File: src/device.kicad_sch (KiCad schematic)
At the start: 68 parts, among them J1 CN-REMO_3W, U1 TLIN14313-Q1, U2 nRF54L10-QDAA, Y1 32MHz, Y2 32.768kHz

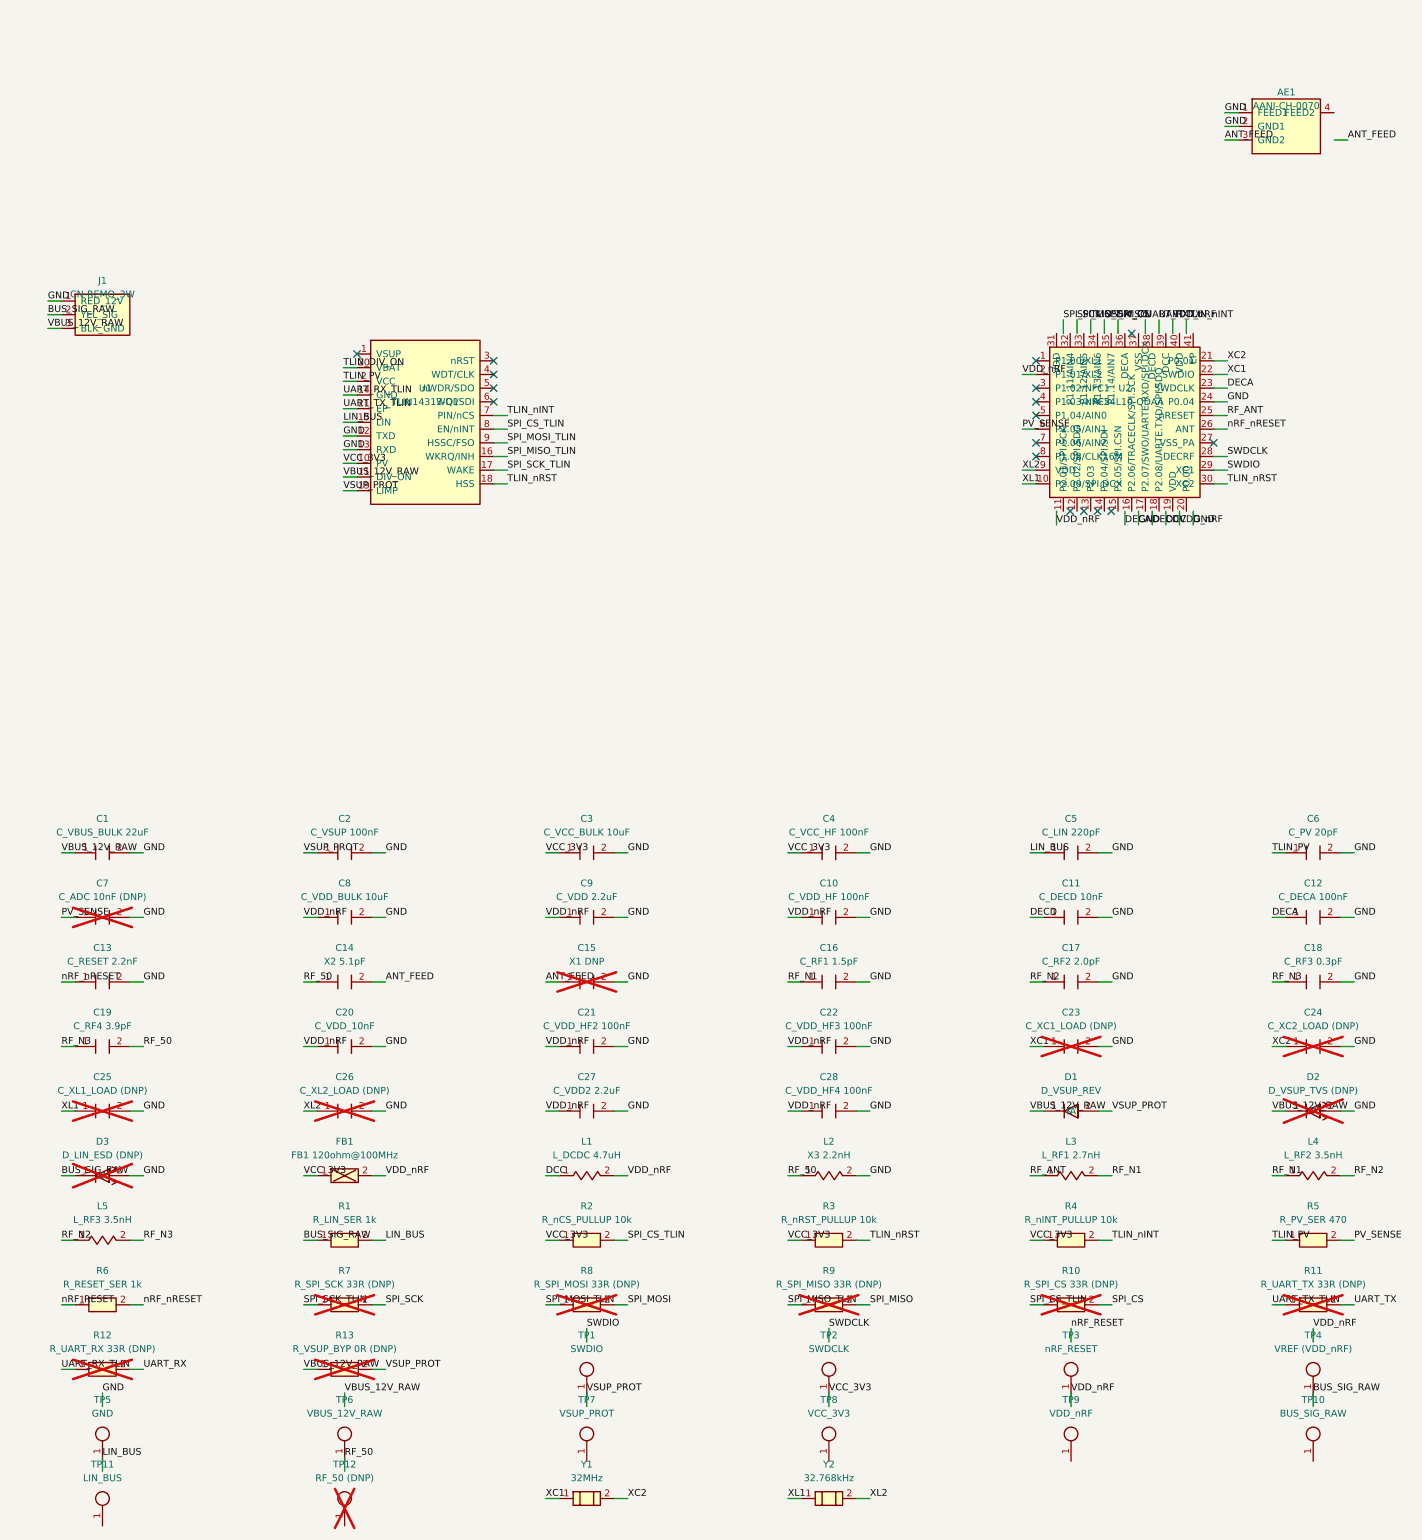
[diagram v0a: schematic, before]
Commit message: stage
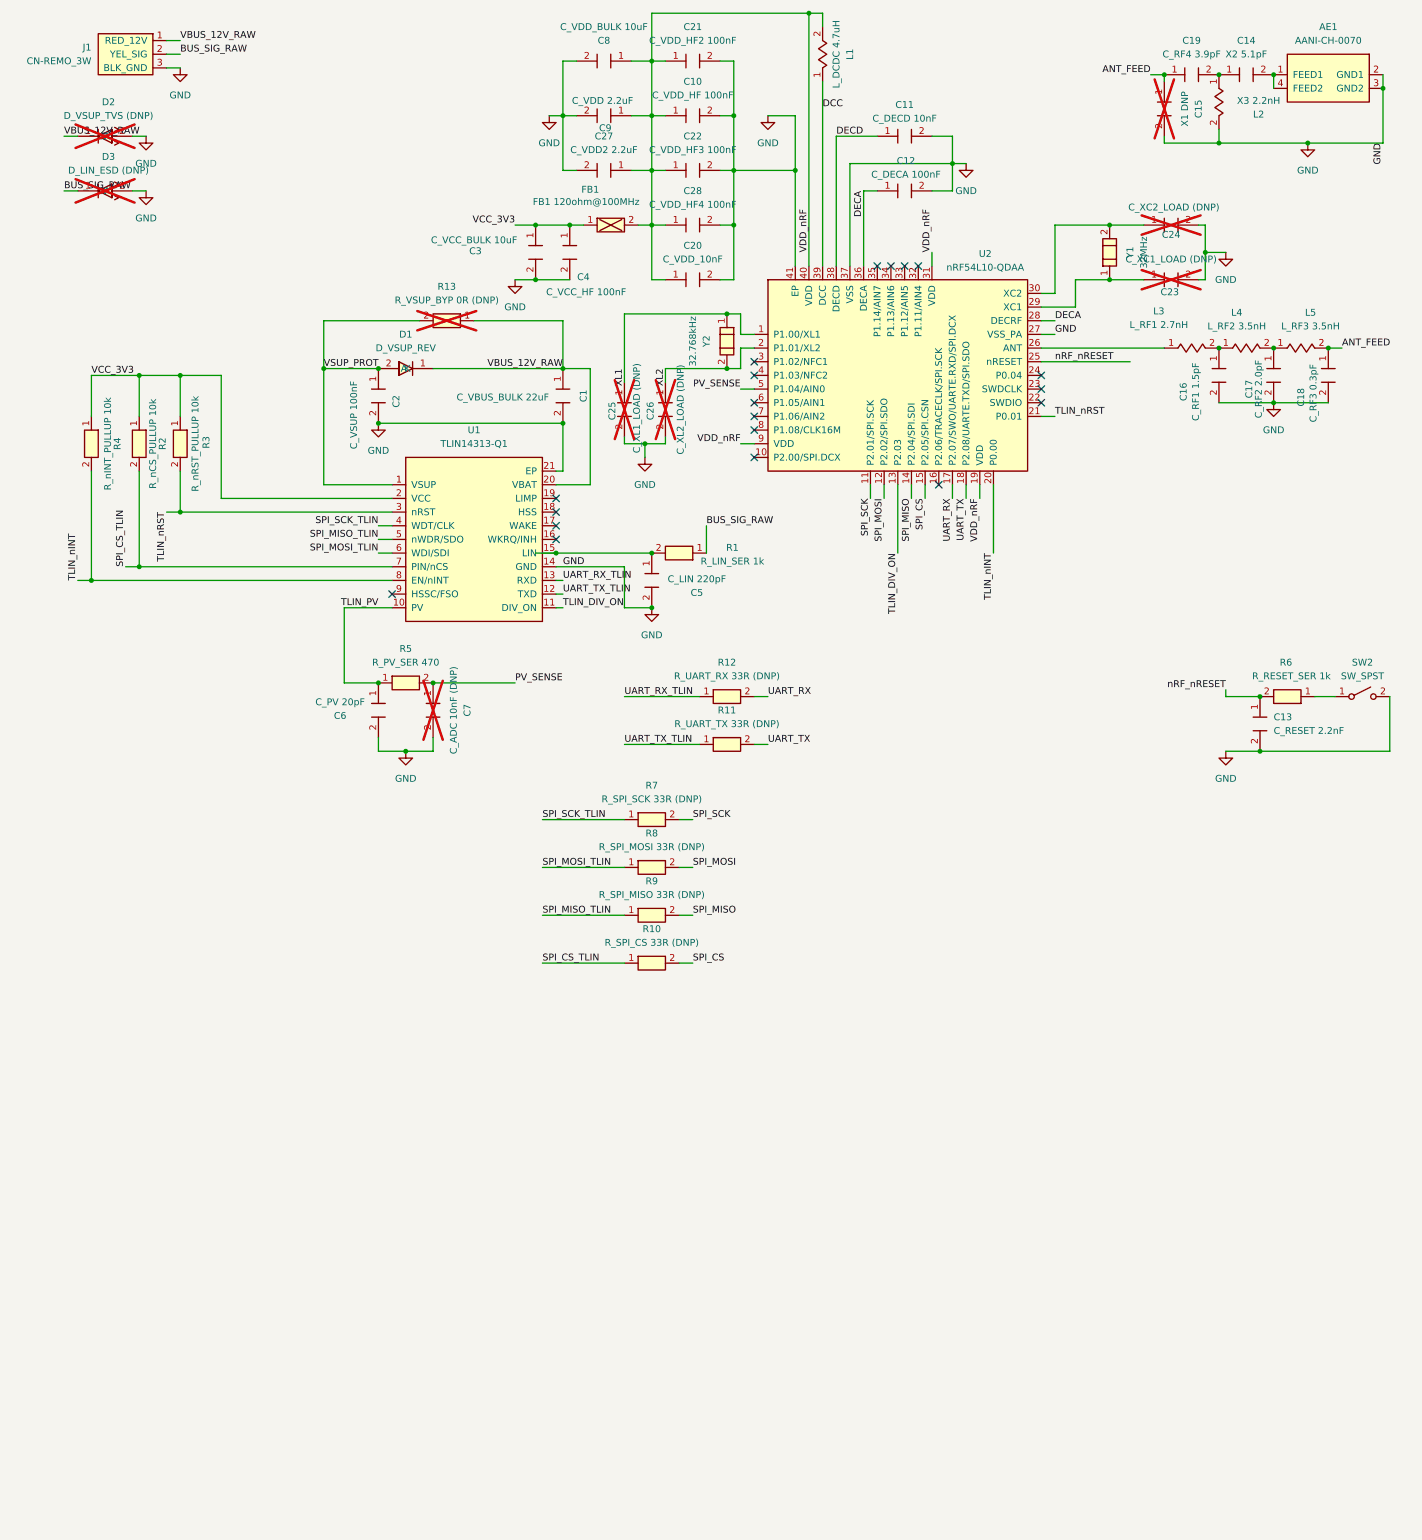
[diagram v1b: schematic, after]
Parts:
- removed TP1: SWDIO, TestPoint:TestPoint_Pad_D1.0mm, symbol device:TestPoint
- removed TP10: BUS_SIG_RAW, TestPoint:TestPoint_Pad_D1.0mm, symbol device:TestPoint
- removed TP11: LIN_BUS, TestPoint:TestPoint_Pad_D1.0mm, symbol device:TestPoint
- removed TP12: RF_50 (DNP), TestPoint:TestPoint_Pad_D1.0mm, symbol device:TestPoint
- removed TP2: SWDCLK, TestPoint:TestPoint_Pad_D1.0mm, symbol device:TestPoint
- removed TP3: nRF_RESET, TestPoint:TestPoint_Pad_D1.0mm, symbol device:TestPoint
- removed TP4: VREF (VDD_nRF), TestPoint:TestPoint_Pad_D1.0mm, symbol device:TestPoint
- removed TP5: GND, TestPoint:TestPoint_Pad_D1.0mm, symbol device:TestPoint
- removed TP6: VBUS_12V_RAW, TestPoint:TestPoint_Pad_D1.0mm, symbol device:TestPoint
- removed TP7: VSUP_PROT, TestPoint:TestPoint_Pad_D1.0mm, symbol device:TestPoint
- removed TP8: VCC_3V3, TestPoint:TestPoint_Pad_D1.0mm, symbol device:TestPoint
- removed TP9: VDD_nRF, TestPoint:TestPoint_Pad_D1.0mm, symbol device:TestPoint
- added SW2: SW_SPST, symbol Switch:SW_SPST
- R10, R11, R12, R7, R8, R9: now fitted
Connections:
- net RF_N3 is gone; now on net ANT_FEED: C18.1, C19.1, L5.2
- net SWDCLK is gone; now on net DECA: U2.28 (DECRF)
- net ANT_FEED: no longer AE1.3 (GND2), C14.2
- net DCC: now also U2.39 (DCC)
- net DECA: now also U2.36 (DECA); no longer U2.23 (SWDCLK)
- net DECD: now also U2.38 (DECD)
- net GND: now also AE1.3 (GND2), J1.3 (BLK_GND), U1.14 (GND), U1.21 (EP), U2.27 (VSS_PA), U2.37 (VSS), U2.41 (EP), SW2.2 (B); no longer AE1.1 (FEED1), J1.1 (RED_12V), U1.12 (TXD), U1.13 (RXD), U2.24 (P0.04)
- net PV_SENSE: now also U2.5 (P1.04/AIN0); no longer U2.6 (P1.05/AIN1)
- net SPI_CS: now also U2.15 (P2.05/SPI.CSN)
- net SPI_CS_TLIN: now also U1.7 (PIN/nCS); no longer U1.8 (EN/nINT)
- net SPI_MISO: now also U2.14 (P2.04/SPI.SDI)
- net SPI_MISO_TLIN: now also U1.5 (nWDR/SDO); no longer U1.16 (WKRQ/INH)
- net SPI_MOSI: now also U2.12 (P2.02/SPI.SDO)
- net SPI_MOSI_TLIN: now also U1.6 (WDI/SDI); no longer U1.9 (HSSC/FSO)
- net SPI_SCK: now also U2.11 (P2.01/SPI.SCK)
- net SPI_SCK_TLIN: now also U1.4 (WDT/CLK); no longer U1.17 (WAKE)
- net TLIN_DIV_ON: now also U1.11 (DIV_ON), U2.13 (P2.03); no longer U1.20 (VBAT)
- net TLIN_PV: now also U1.10 (PV); no longer U1.2 (VCC)
- net TLIN_nINT: now also U1.8 (EN/nINT), U2.20 (P0.00); no longer U1.7 (PIN/nCS)
- net TLIN_nRST: now also U1.3 (nRST), U2.21 (P0.01); no longer U1.18 (HSS), U2.30 (XC2)
- net UART_RX: now also U2.17 (P2.07/SWO/UARTE.RXD/SPI.DCX)
- net UART_RX_TLIN: now also U1.13 (RXD); no longer U1.14 (GND)
- net UART_TX: now also U2.18 (P2.08/UARTE.TXD/SPI.SDO)
- net UART_TX_TLIN: now also U1.12 (TXD); no longer U1.21 (EP)
- net VBUS_12V_RAW: now also J1.1 (RED_12V), U1.20 (VBAT); no longer J1.3 (BLK_GND), U1.11 (DIV_ON)
- net VCC_3V3: now also U1.2 (VCC); no longer U1.10 (PV)
- net VDD_nRF: now also U2.19 (VDD), U2.31 (VDD), U2.40 (VDD), U2.9 (VDD); no longer U2.2 (P1.01/XL2)
- net VSUP_PROT: now also U1.1 (VSUP); no longer U1.19 (LIMP)
- net XL1: now also U2.1 (P1.00/XL1); no longer U2.10 (P2.00/SPI.DCX)
- net XL2: now also U2.2 (P1.01/XL2); no longer U2.9 (VDD)
- net nRF_nRESET: now also U2.25 (nRESET); no longer U2.26 (ANT)
- net at AE1.4 (FEED2): now also AE1.1 (FEED1), C14.2
- net LIN_BUS: no longer names the net of C5.1, R1.2, U1.15 (LIN)
- net RF_50: no longer names the net of C14.1, C19.2, L2.1
- net RF_ANT: no longer names the net of L3.1
- net RF_ANT: now also U2.26 (ANT); no longer U2.25 (nRESET)
- net RF_N1: no longer names the net of C16.1, L3.2, L4.1
- net RF_N2: no longer names the net of C17.1, L4.2, L5.1
- net SWDIO: no longer names the net of U2.29 (XC1)
- net SWDIO: now also C23.1, Y1.1
- removed net XC1: C23.1, U2.22 (SWDIO), Y1.1
- net XC2: no longer names the net of C24.1, Y1.2
- net XC2: now also U2.30 (XC2); no longer U2.21 (P0.01)
- net nRF_RESET: no longer names the net of R6.1
- net nRF_RESET: now also SW2.1 (A)
- no-connect marks 17 -> 19
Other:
- moved on the sheet: AE1, C1, C10, C11, C12, C13, C14, C15, C16, C17, C18, C19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
